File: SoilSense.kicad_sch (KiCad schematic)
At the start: 22 parts, among them J3 OSTVN04A150, Q5 PMH950UPEH, U4 SN75176BDR, U8 74HC04D

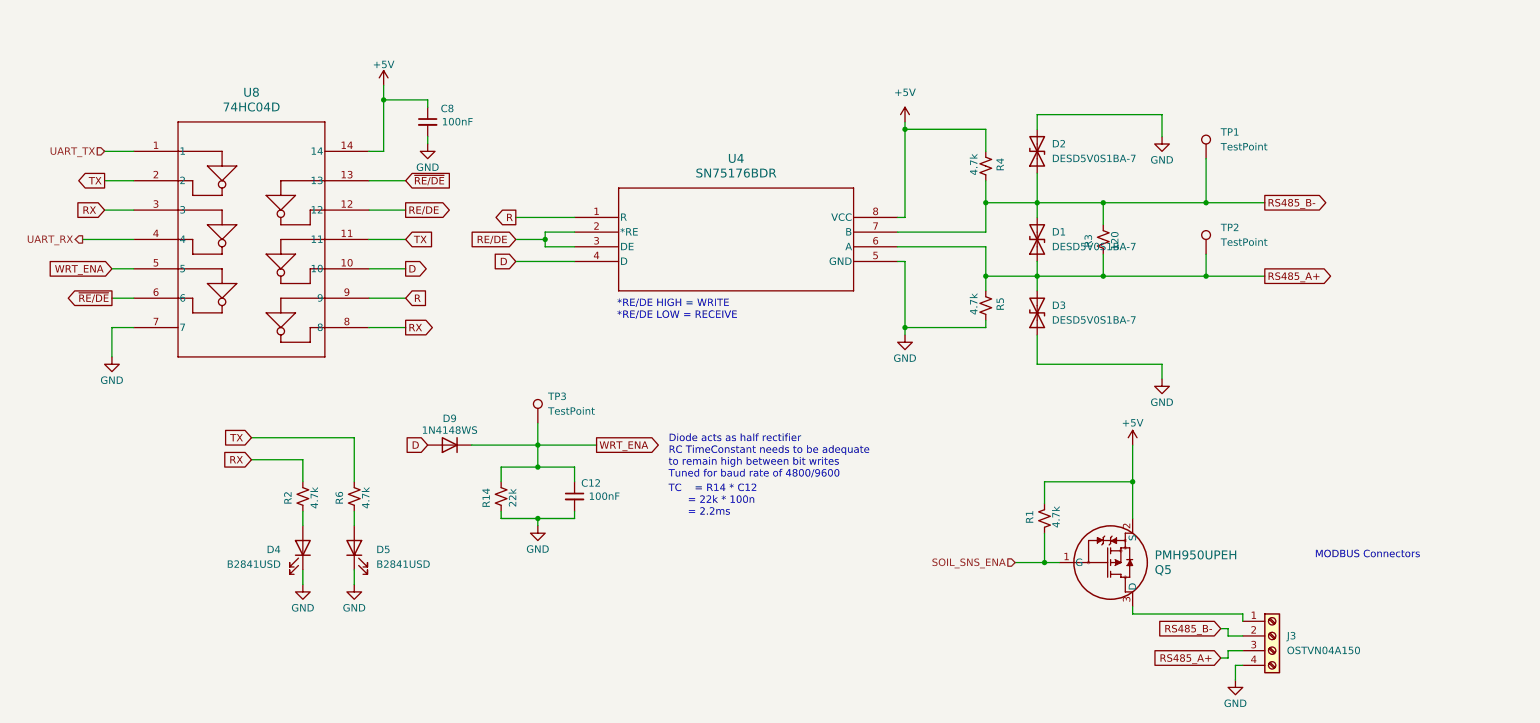
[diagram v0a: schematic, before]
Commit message: 2nd rev schematic done
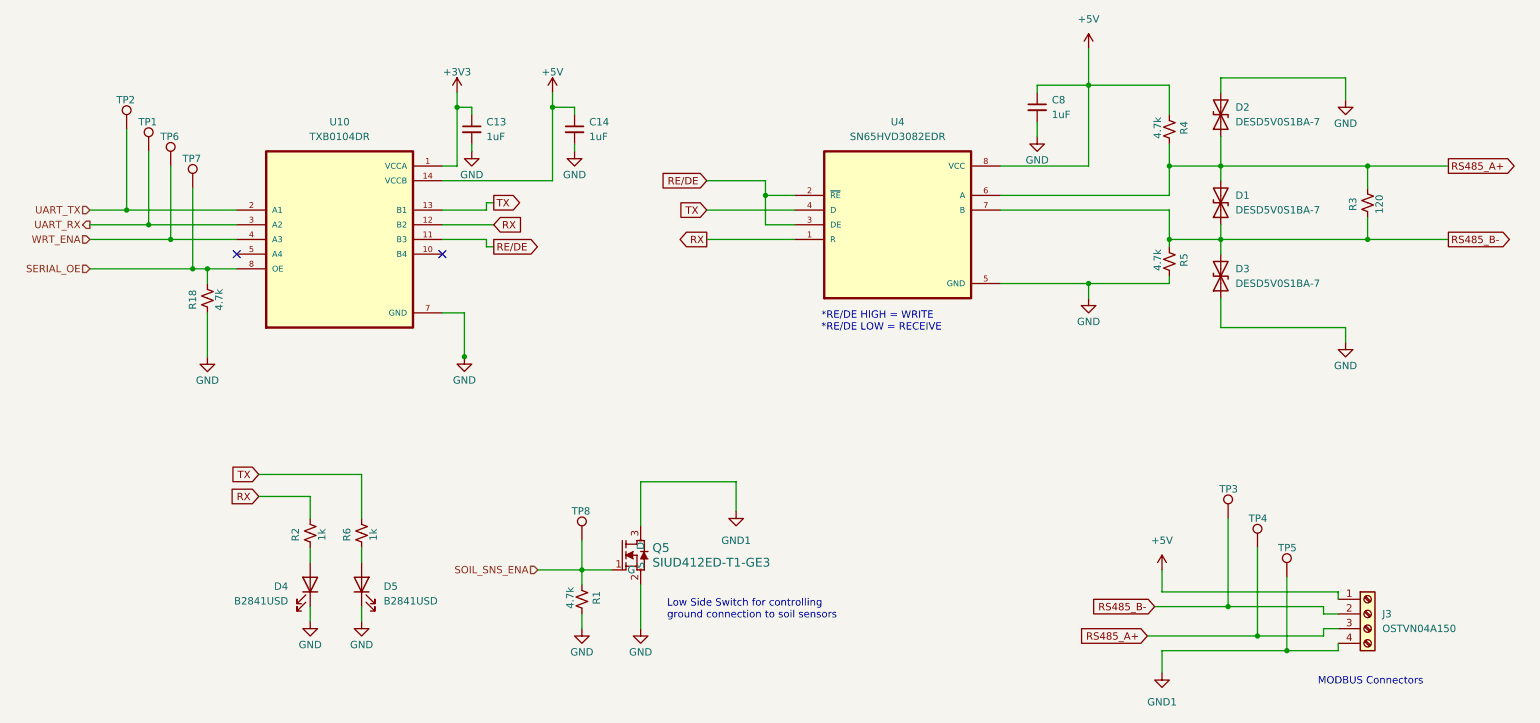
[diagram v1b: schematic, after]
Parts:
- removed C12: 100nF, Capacitor_SMD:C_0402_1005Metric, symbol Device:C_Small
- removed D9: 1N4148WS, Diode_SMD:D_SOD-323, symbol Diode:1N4148WS
- removed Q5: PMH950UPEH, SproutSenseFootprints:QPMOS1G2S3d_SOT8001_NEX, symbol SproutSense:PMH950UPEH
- removed R14: 22k, Resistor_SMD:R_0402_1005Metric, symbol Device:R_Small_US
- removed U4: SN75176BDR, Package_SO:SOP-8_3.76x4.96mm_P1.27mm, symbol SproutSense:SN75176BDR
- removed U8: 74HC04D, Package_SO:SOIC-14_3.9x8.7mm_P1.27mm, symbol SproutSense:74HC04D
- added C13, C14: 1uF, Capacitor_SMD:C_0402_1005Metric, symbol Device:C_Small
- added Q5: SIUD412ED-T1-GE3, SMT_412ED-T1-GE3_VIS, symbol SproutSense:SIUD412ED-T1-GE3
- added R18: 4.7k, Resistor_SMD:R_0402_1005Metric, symbol Device:R_Small_US
- added TP4, TP5, TP6, TP7, TP8: TestPoint, symbol Connector:TestPoint
- added U10: TXB0104DR, SproutSenseFootprints:SOIC127P600X175-14N, symbol SproutSense:TXB0104DR
- added U4: SN65HVD3082EDR, SproutSenseFootprints:SOIC127P599X175-8N, symbol SproutSense:SN65HVD3082EDR
- C8: value 100nF -> 1uF; Distributor Prt # 1276-1002-1-ND -> 490-10024-1-ND - Cut Tape (CT); Manuf Prt # CL05B104KP5NNNC -> GRM155R70J105KA12D
- R2, R6: value 4.7k -> 1k; Distributor Prt # 311-4.7KJRCT-ND -> 311-1.0KJRCT-ND; Manuf Prt # RC0402JR-074K7L -> RC0402JR-071KL
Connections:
- net +5V: now also J3.1 (Pin_1), C14.1, U10.14 (VCCB), U4.8 (VCC); no longer R1.2
- net GND: now also R1.1, C13.2, C14.2, Q5.2 (S), R18.2, U10.7 (GND), U4.5 (GND); no longer J3.4 (Pin_4)
- net RE/DE: now also U10.11 (B3), U4.2 (~{RE}), U4.3 (DE)
- net RS485_A+: now also D1.2 (A2), D2.1 (A1), R3.1, R4.1, TP4.1, U4.6 (A); no longer D1.1 (A1), D3.2 (A2), R3.2, R5.2, TP2.1
- net RS485_B-: now also D1.1 (A1), D3.2 (A2), R3.2, R5.2, TP3.1, U4.7 (B); no longer D1.2 (A2), D2.1 (A1), R3.1, R4.1, TP1.1
- net RX: now also U10.12 (B2), U4.1 (R)
- net SOIL_SNS_ENA: now also R1.2, Q5.1 (G), TP8.1; no longer R1.1
- net TX: now also U10.13 (B1), U4.4 (D)
- net UART_RX: now also TP1.1, U10.3 (A2)
- net UART_TX: now also TP2.1, U10.2 (A1)
- net WRT_ENA: now also TP6.1, U10.4 (A3); no longer TP3.1
- new net +3V3: C13.1, U10.1 (VCCA)
- new net GND1: J3.4 (Pin_4), Q5.3 (D), TP5.1
- new net SERIAL_OE: R18.1, TP7.1, U10.8 (OE)
- no-connect marks 0 -> 2
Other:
- note added: "Low Side Switch for controlling ground connection to soil sensors"
- note removed: "Diode acts as half rectifier RC TimeConstant needs to be adequate to remain high between bit writes Tuned for baud rate of 4800/9600"
- note removed: "TC = R14 * C12 = 22k * 100n = 2.2ms"
- moved on the sheet: D1, D2, D3, D4, D5, J3, R3, R4, R5
